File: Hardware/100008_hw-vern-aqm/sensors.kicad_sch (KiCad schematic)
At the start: 8 parts

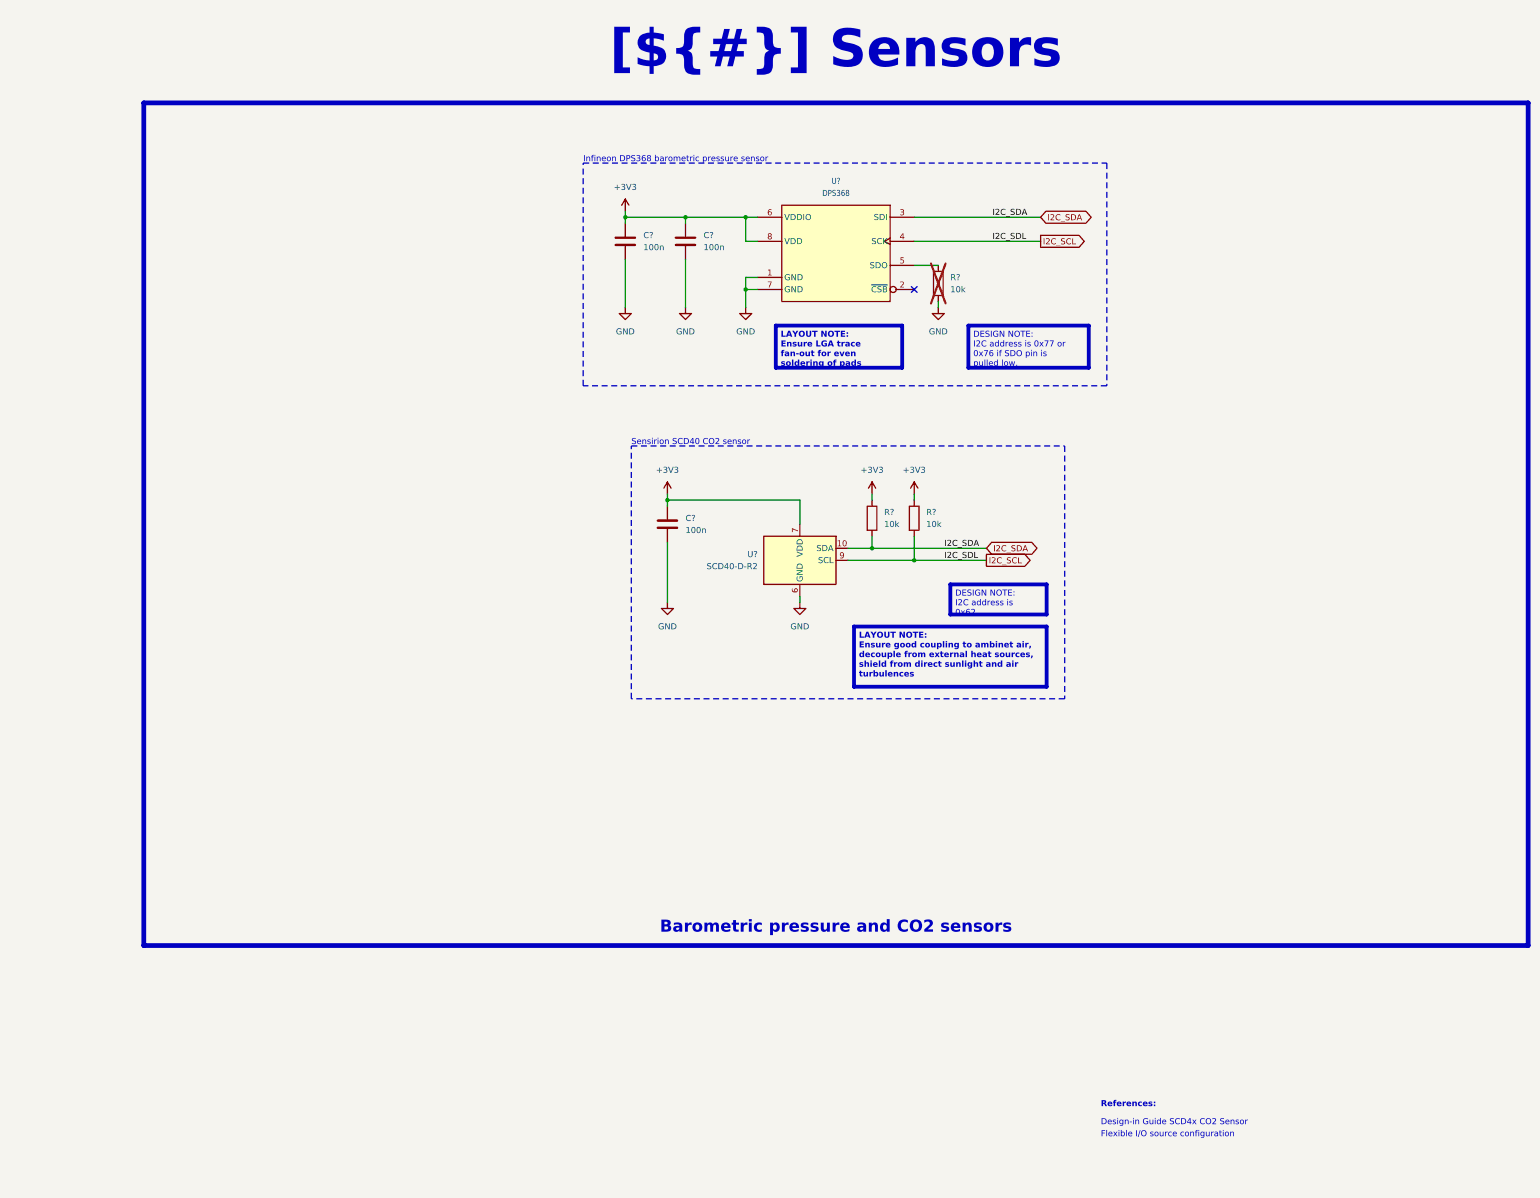
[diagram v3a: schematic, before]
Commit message: schematic and pcb layout
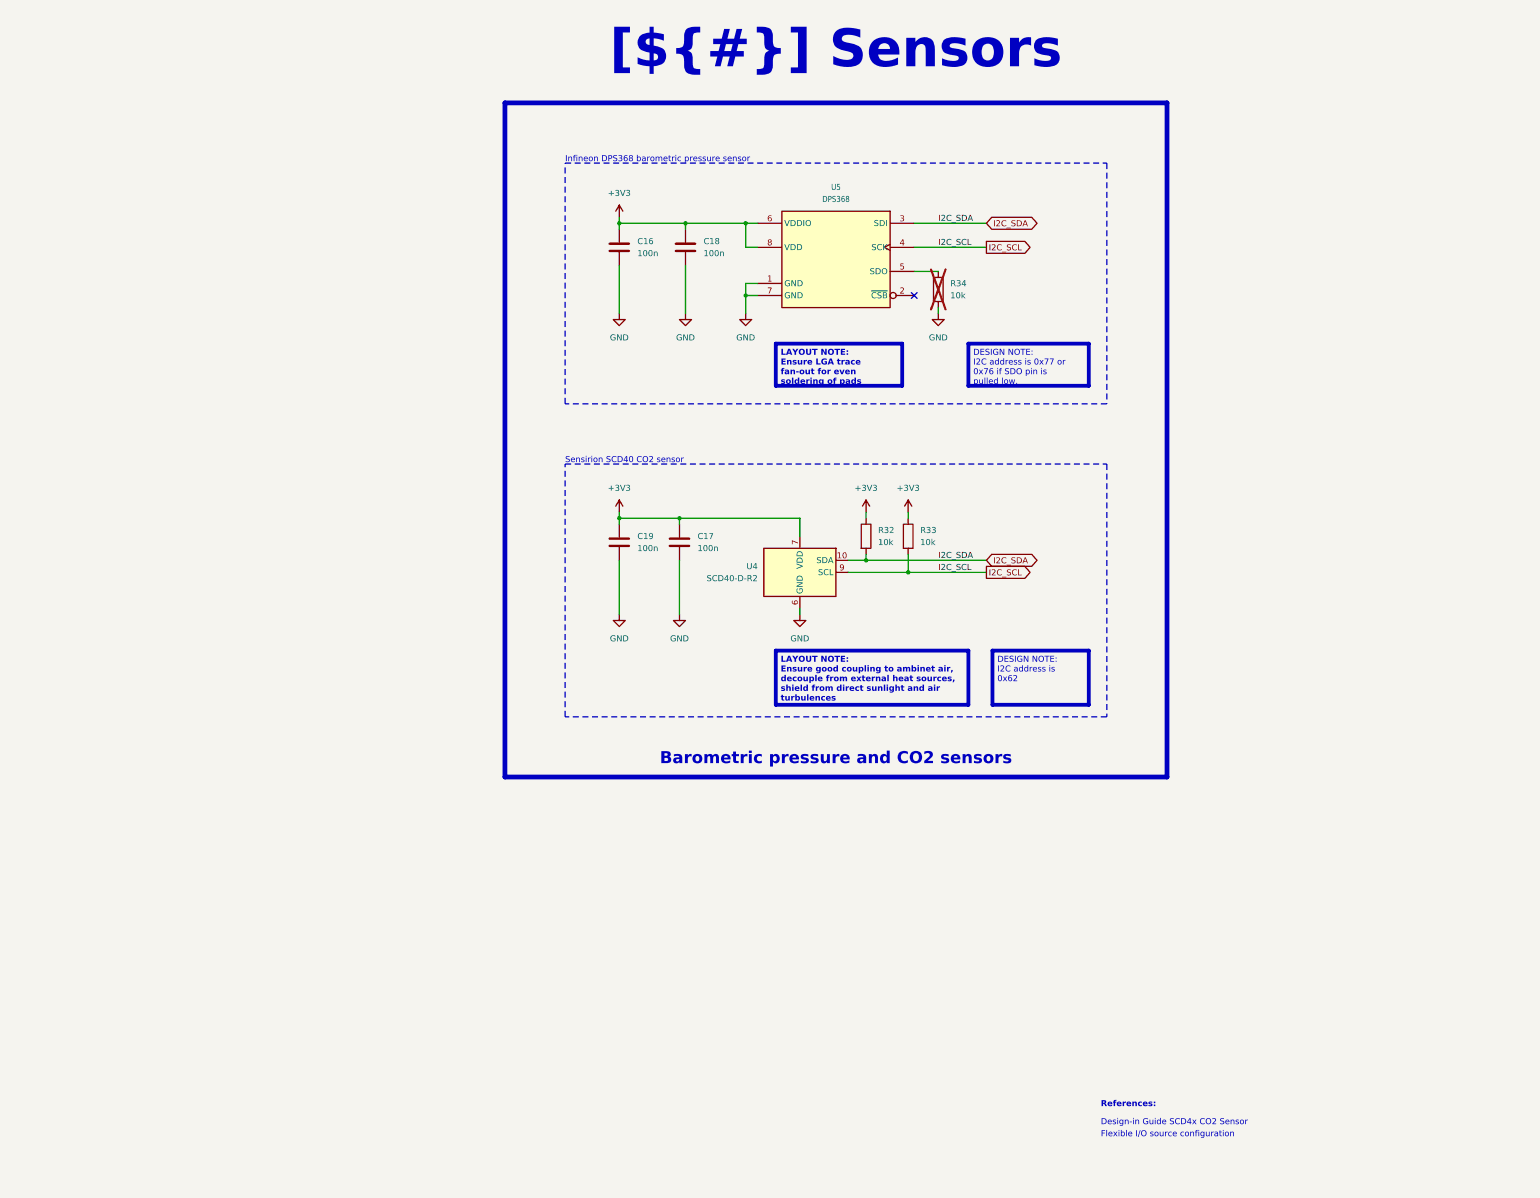
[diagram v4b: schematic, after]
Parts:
- added C19: 100n, Capacitor_SMD:C_0603_1608Metric, symbol Device:C
- gave numbers to parts that had none: 8
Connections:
- net +3V3: now also C19.1
- net GND: now also C19.2
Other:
- moved on the sheet: C16, C17, C18, R32, R33, R34, U4, U5
